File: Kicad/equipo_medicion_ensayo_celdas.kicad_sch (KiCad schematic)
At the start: 2 parts, among them J1 Conn_01x12, U2 STM32WB55RGVx

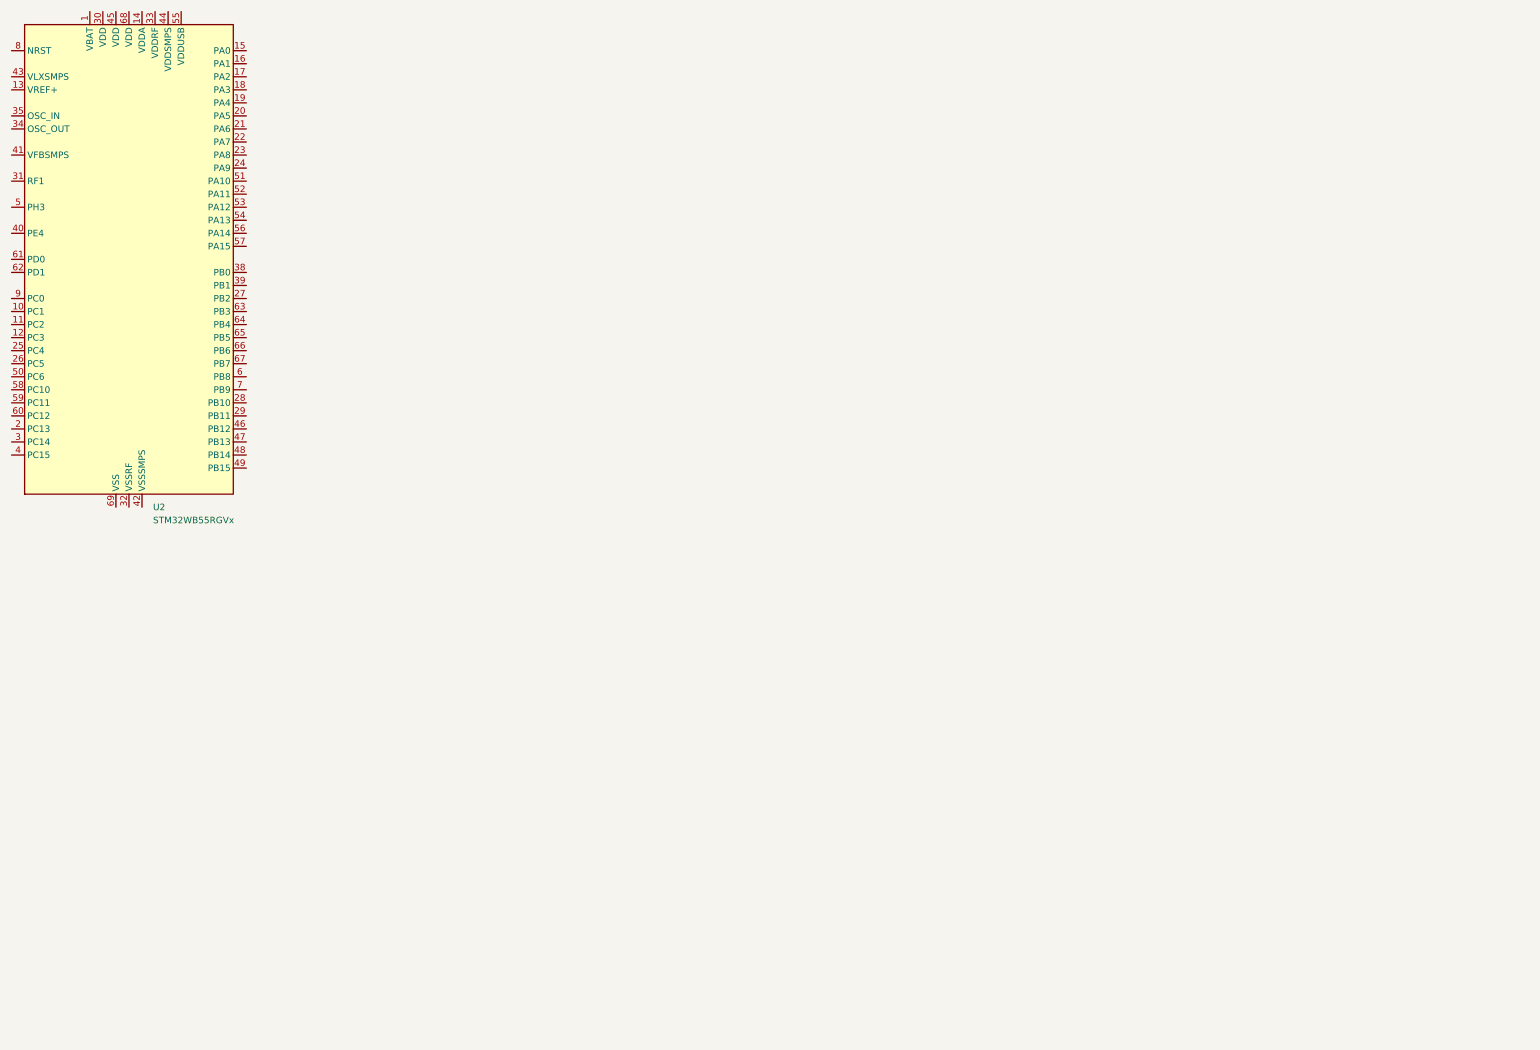
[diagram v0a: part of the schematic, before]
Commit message: Más avances en esquemático de Kicad.
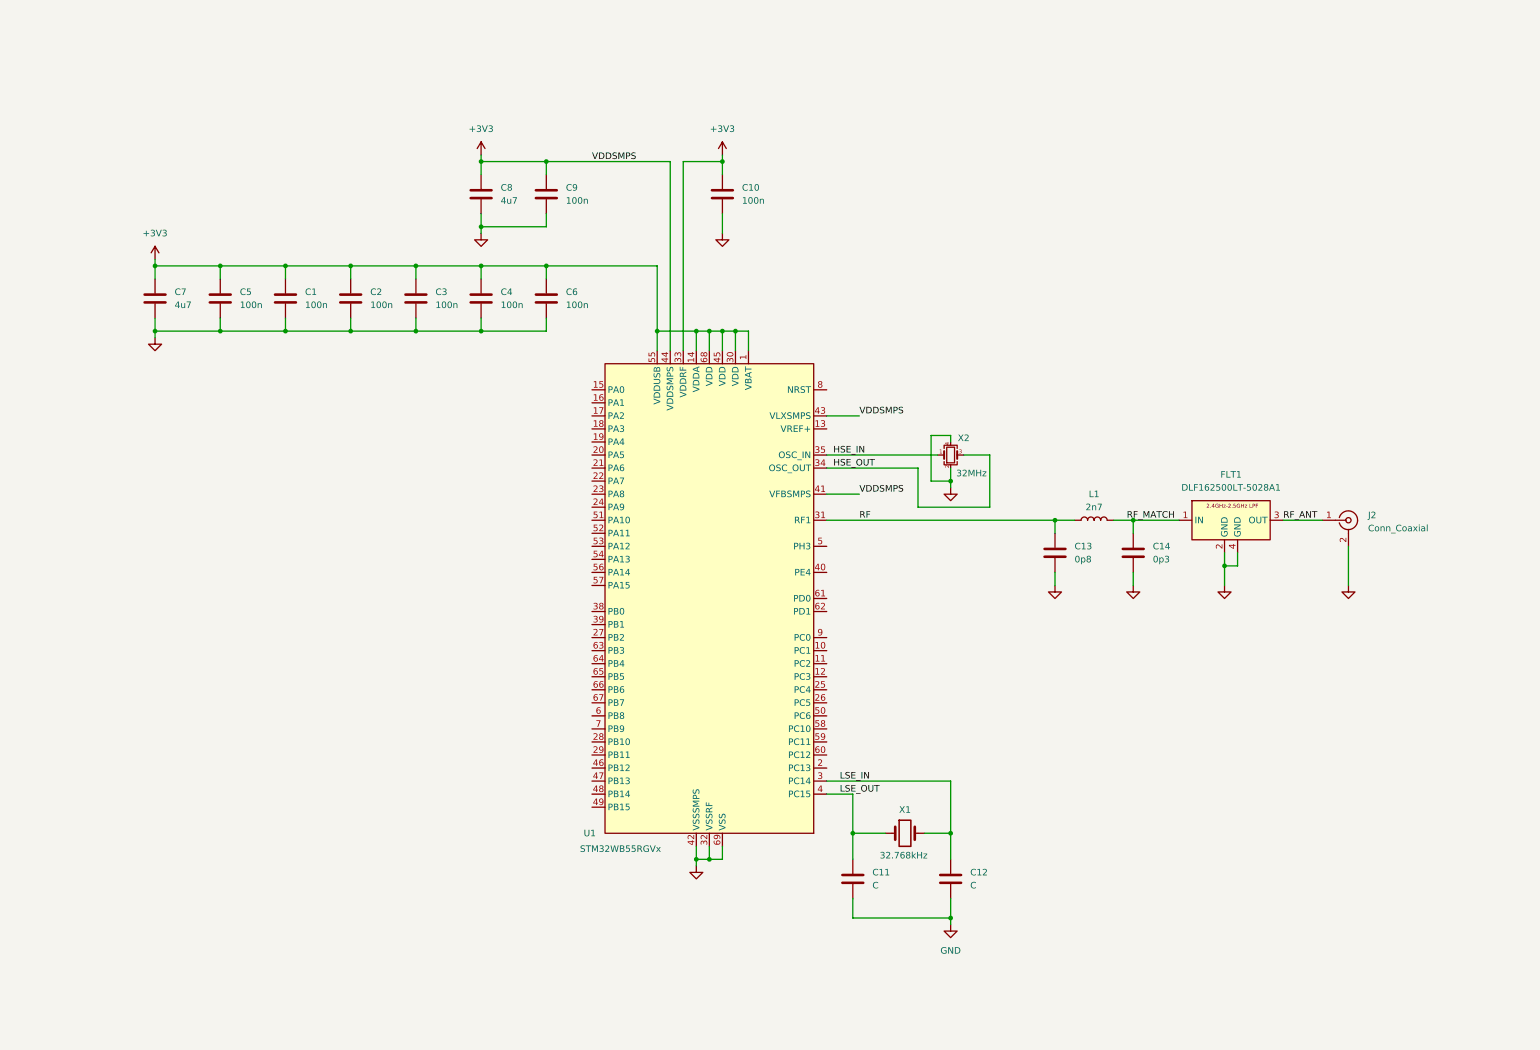
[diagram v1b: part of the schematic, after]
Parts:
- added C1, C10, C2, C3, C4, C5, C6, C9: 100n, symbol Device:C
- added C11, C12: C, symbol Device:C
- added C13: 0p8, symbol Device:C
- added C14: 0p3, symbol Device:C
- added C7, C8: 4u7, symbol Device:C
- added FLT1: DLF162500LT-5028A1, equipo_medicion_ensayo_celdas_footprints:DLF162500LT-5028A1, symbol equipo_medicion_ensayo_celdas_sch_symbols:DLF162500LT-5028A1
- added J2: Conn_Coaxial, symbol Connector:Conn_Coaxial
- added L1: 2n7, symbol Device:L
- added X1: 32.768kHz, symbol Device:Crystal
- added X2: 32MHz, symbol Device:Crystal_GND24_Small
- renumbered U2 to U1
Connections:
- net +3V3: now also U1.1 (VBAT), U1.14 (VDDA), U1.30 (VDD), U1.33 (VDDRF), U1.41 (VFBSMPS), U1.43 (VLXSMPS), U1.44 (VDDSMPS), U1.45 (VDD), U1.55 (VDDUSB), U1.68 (VDD), C1.1, C10.1, C2.1, C3.1, C4.1, C5.1, C6.1, C7.1, C8.1, C9.1
- net GND: now also U1.32 (VSSRF), U1.42 (VSSSMPS), U1.69 (VSS), C1.2, C10.2, C11.2, C12.2, C13.2, C14.2, C2.2, C3.2, C4.2, C5.2, C6.2, C7.2, C8.2, C9.2, FLT1.2 (GND), FLT1.4 (GND), J2.2 (Ext), X2.2, X2.4
- net LSE_IN: now reaches U1.3 (PC14)
- net LSE_IN: now also C12.1, X1.2
- net RF: now reaches U1.31 (RF1)
- net RF: now also C13.1, L1.1
- net HSE_OUT: now reaches U1.34 (OSC_OUT)
- net HSE_OUT: now also X2.3
- net HSE_IN: now reaches U1.35 (OSC_IN)
- net HSE_IN: now also X2.1
- net LSE_OUT: now reaches U1.4 (PC15)
- net LSE_OUT: now also C11.1, X1.1
- new net RF_ANT: FLT1.3 (OUT), J2.1 (In)
- new net RF_MATCH: C14.1, FLT1.1 (IN), L1.2
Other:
- moved on the sheet: U1
